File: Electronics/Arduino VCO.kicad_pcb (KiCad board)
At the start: 2 copper layers, 61 parts, among them J5 Conn_02x08_Odd_Even, U1 TL072

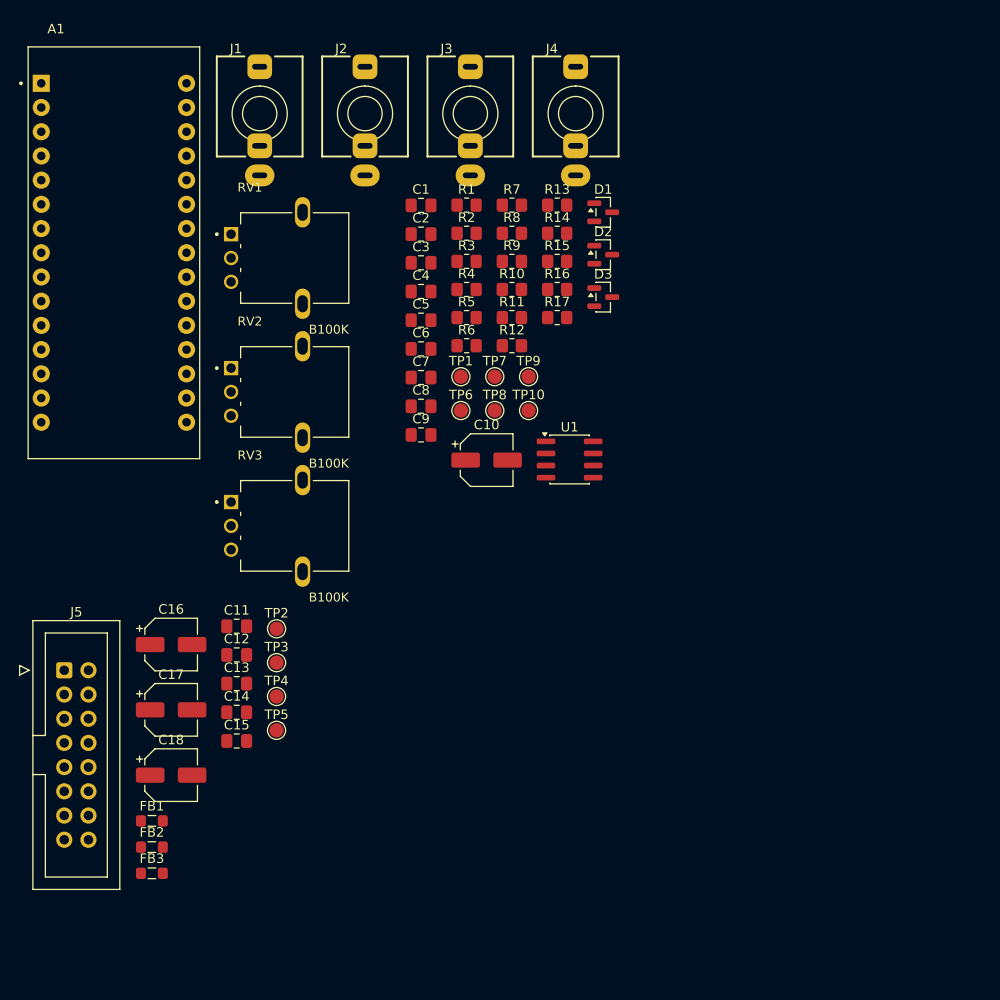
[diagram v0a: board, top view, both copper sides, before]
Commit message: deleting unused files
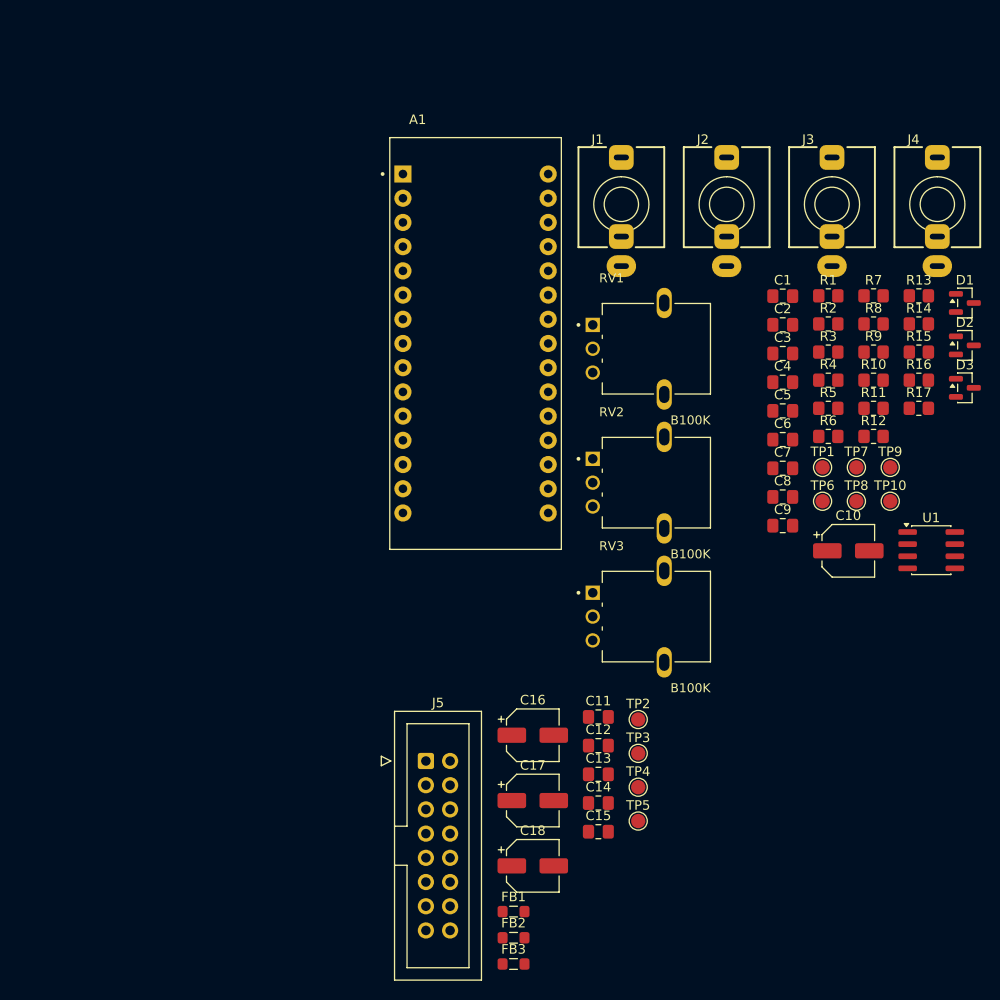
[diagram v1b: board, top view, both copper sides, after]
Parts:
- moved R1 39.1 mm to (115.6, 57.1)
- moved R10 39.1 mm to (120.3, 65.9)
- moved R11 39.1 mm to (120.3, 68.9)
- moved R12 39.1 mm to (120.3, 71.8)
- moved R13 39.1 mm to (125.1, 57.1)
- moved R14 39.1 mm to (125.1, 60.0)
- moved R15 39.1 mm to (125.1, 63.0)
- moved R16 39.1 mm to (125.1, 65.9)
- moved R17 39.1 mm to (125.1, 68.9)
- moved R2 39.1 mm to (115.6, 60.0)
- moved R3 39.1 mm to (115.6, 63.0)
- moved R4 39.1 mm to (115.6, 65.9)
- moved R5 39.1 mm to (115.6, 68.9)
- moved R6 39.1 mm to (115.6, 71.8)
- moved R7 39.1 mm to (120.3, 57.1)
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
